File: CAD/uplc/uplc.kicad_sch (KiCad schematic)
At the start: 34 parts, among them J1 Conn_01x06_Pin, J2 SM12B-GHS-TB(LF)(SN), K1 G6K-2F-Y, K2 G6K-2F-Y, U1 DS8242-33S5, U3 ESP32-C3-WROOM-02, U5 TBD62003AFWG, Y1 32.568khz 3.2x1.5 12.5pf

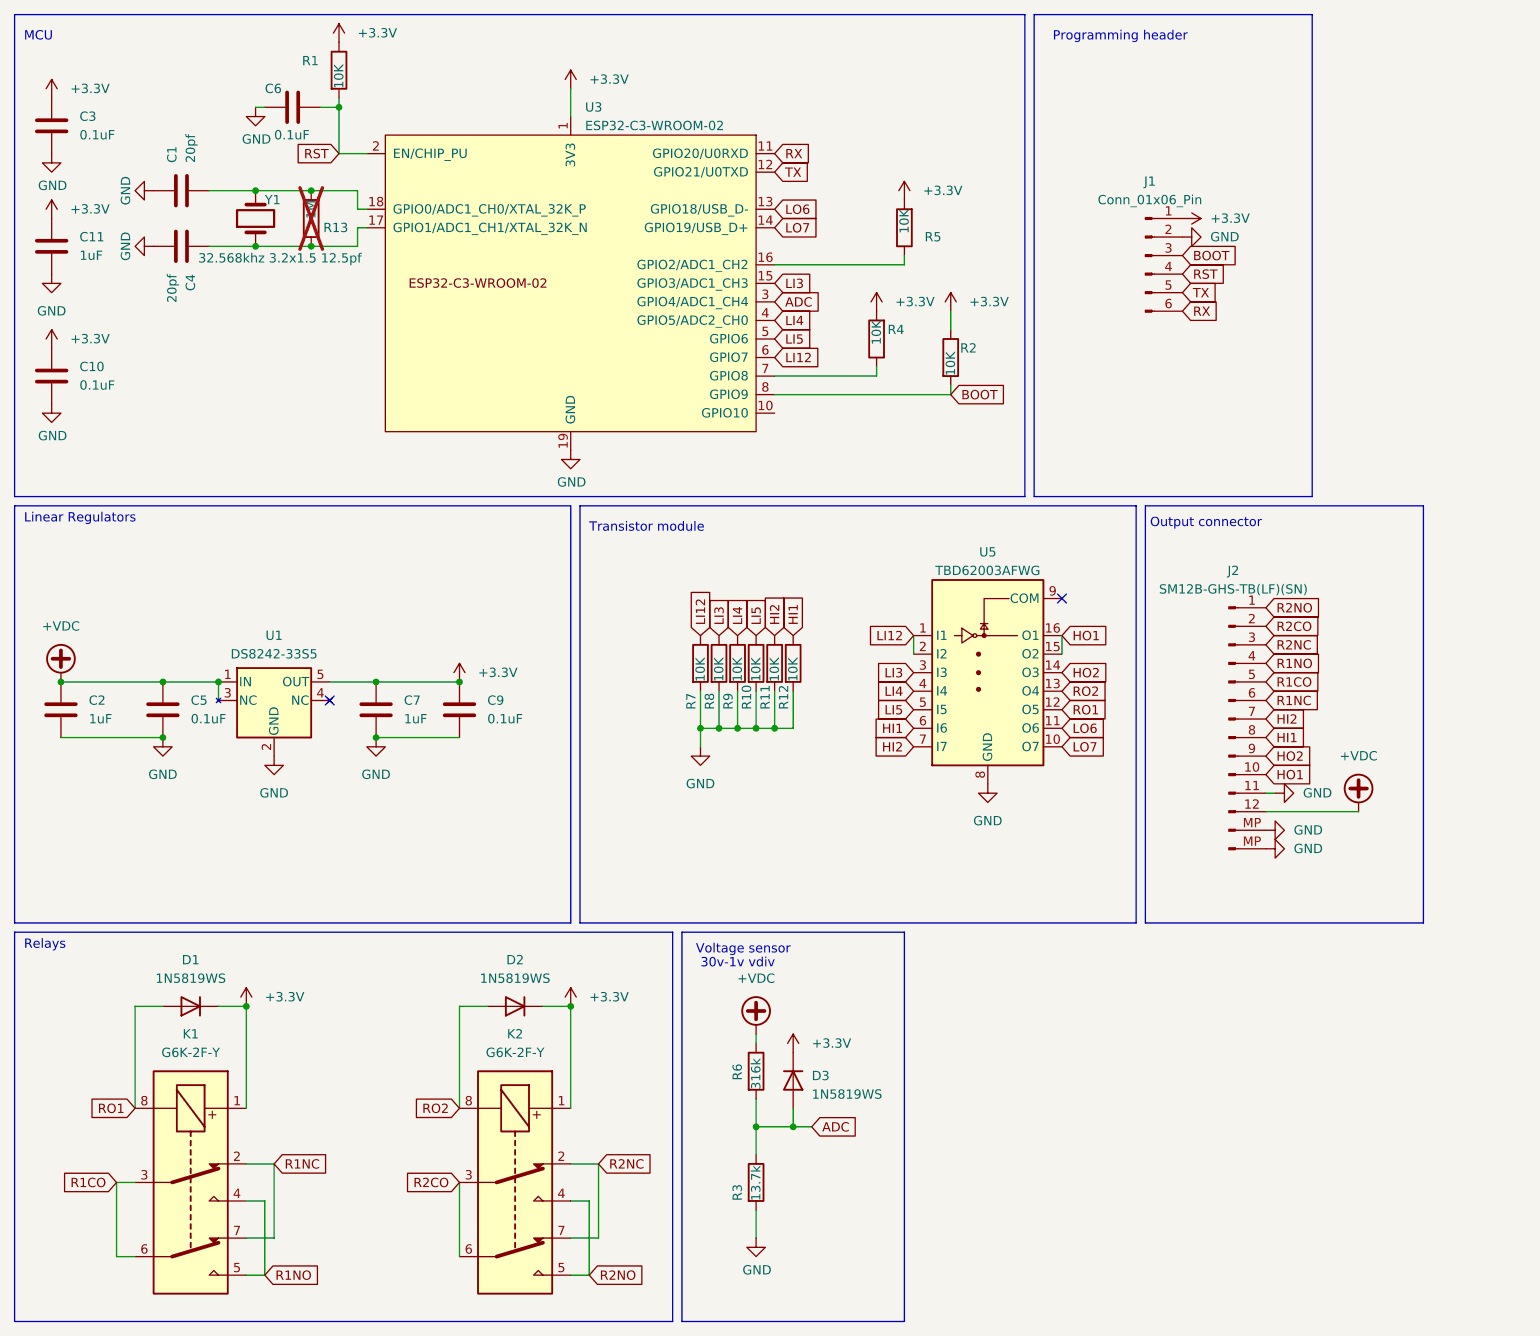
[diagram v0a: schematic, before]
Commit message: rev 1.1
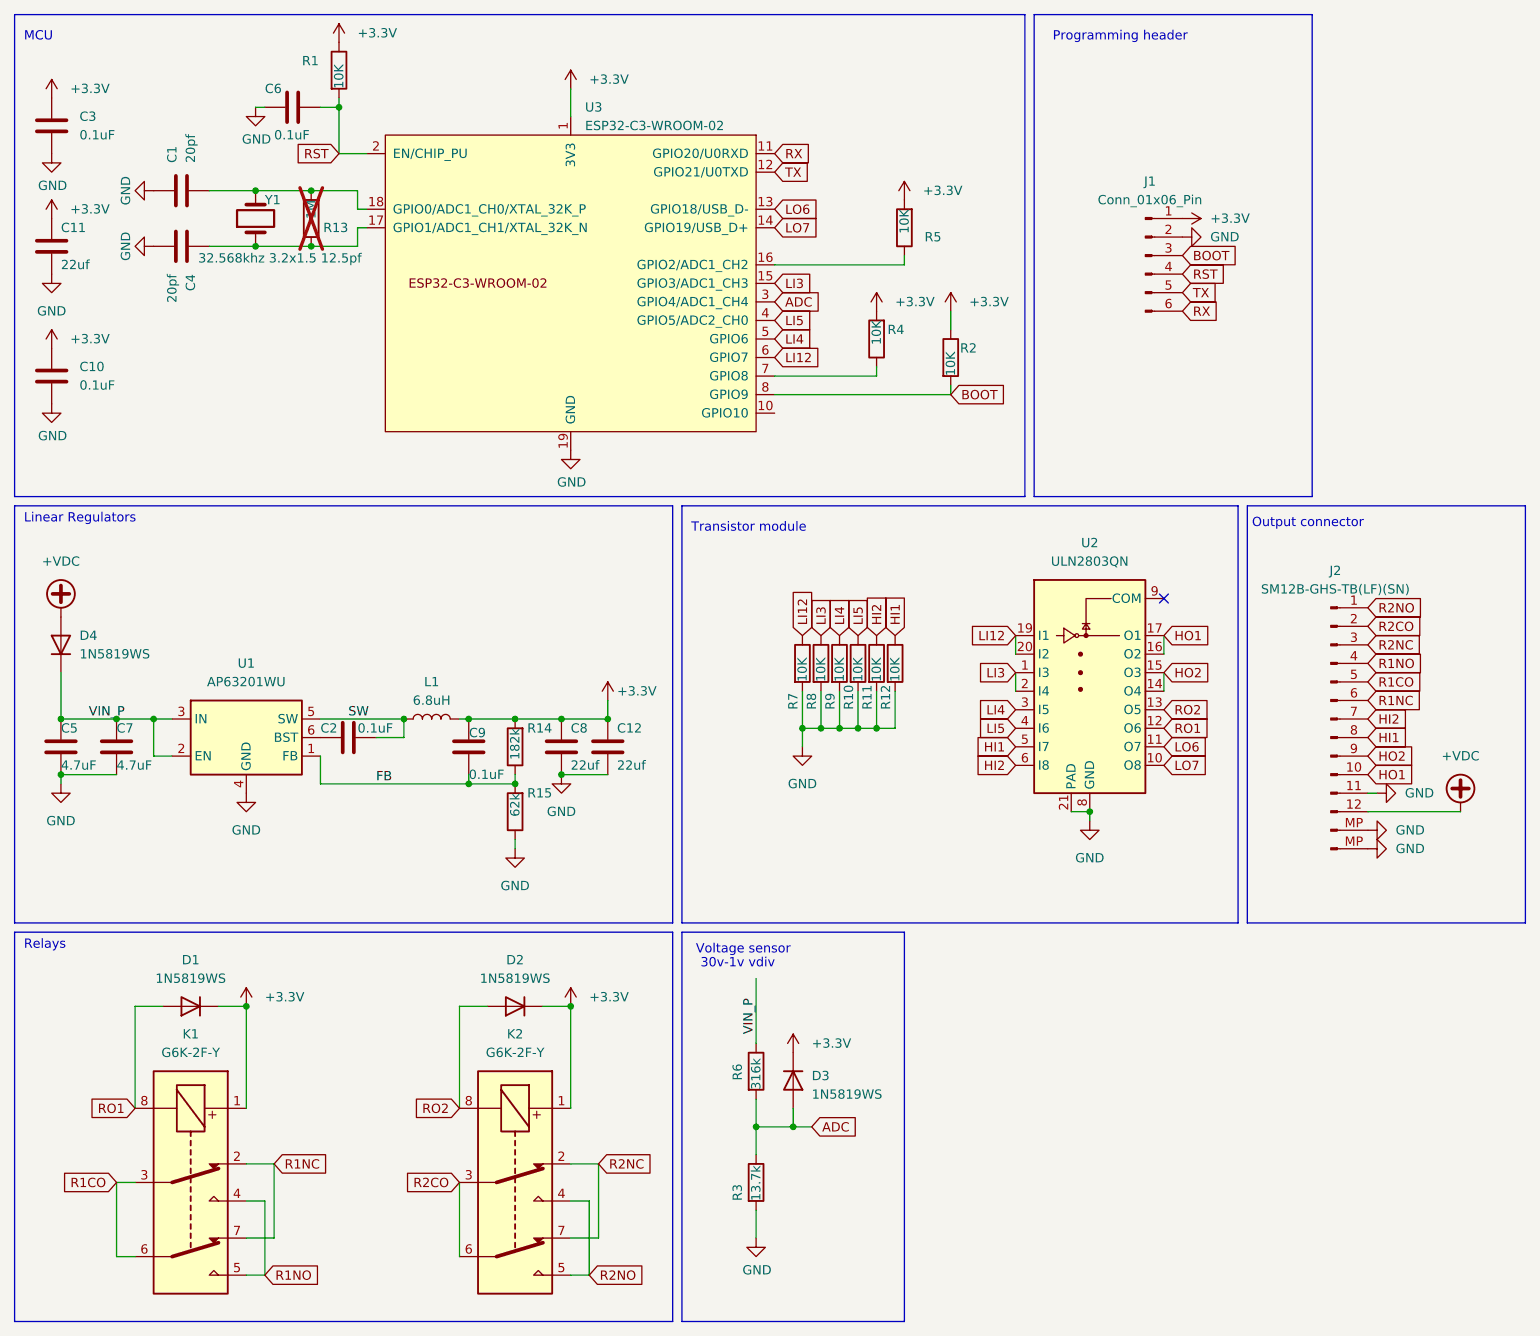
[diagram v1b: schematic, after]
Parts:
- removed U1: DS8242-33S5, Package_TO_SOT_SMD:SOT-23-5, symbol Library:DS8242
- removed U5: TBD62003AFWG, Package_SO:SOIC-16_3.9x9.9mm_P1.27mm, symbol Library:ULN2003A
- added C12, C8: 22uf, Capacitor_SMD:C_0402_1005Metric, symbol Library:C
- added D4: 1N5819WS, Diode_SMD:D_SOD-323, symbol Library:1N4148WS
- added L1: 6.8uH, Inductor_SMD:L_1008_2520Metric, symbol Device:L
- added R14: 182k, Resistor_SMD:R_0402_1005Metric, symbol Library:R
- added R15: 62k, Resistor_SMD:R_0402_1005Metric, symbol Library:R
- added U1: AP63201WU, Package_TO_SOT_SMD:TSOT-23-6, symbol Regulator_Switching:AP63201WU
- added U2: ULN2803QN, Package_DFN_QFN:QFN-20-1EP_4x4mm_P0.5mm_EP2.6x2.6mm, symbol Library:ULN2803QN
- C11: value 1uF -> 22uf; LCSC Part # C52923 -> C415703
- C2: value 1uF -> 0.1uF; LCSC Part # C52923 -> C307331
- C5: value 0.1uF -> 4.7uF; footprint Capacitor_SMD:C_0402_1005Metric -> Capacitor_SMD:C_0603_1608Metric
- C7: value 1uF -> 4.7uF; footprint Capacitor_SMD:C_0402_1005Metric -> Capacitor_SMD:C_0603_1608Metric; LCSC Part # C52923 -> C307331
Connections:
- net +3.3V: now also C12.1, C8.1, L1.2, R14.2; no longer C7.1
- net +VDC: now also D4.2 (A); no longer C2.1, C5.2, R6.1
- net GND: now also C5.2, C12.2, C8.2, R15.1, U1.4 (GND), U2.21 (PAD), U2.8 (GND); no longer C2.2, C5.1, C9.2
- net HI1: now also U2.5 (I7)
- net HI2: now also U2.6 (I8)
- net HO1: now also U2.16 (O2), U2.17 (O1)
- net HO2: now also U2.14 (O4), U2.15 (O3)
- net LI12: now also U2.19 (I1), U2.20 (I2)
- net LI3: now also U2.1 (I3), U2.2 (I4)
- net LI4: now also U3.5 (GPIO6), U2.3 (I5); no longer U3.4 (GPIO5/ADC2_CH0)
- net LI5: now also U3.4 (GPIO5/ADC2_CH0), U2.4 (I6); no longer U3.5 (GPIO6)
- net LO6: now also U2.11 (O7)
- net LO7: now also U2.10 (O8)
- net RO1: now also U2.12 (O6)
- net RO2: now also U2.13 (O5)
- new net: C2.2, U1.6 (BST)
- new net FB: C9.2, R14.1, R15.2, U1.1 (FB)
- new net SW: C2.1, L1.1, U1.5 (SW)
- new net VIN_P: C5.1, C7.1, D4.1 (K), R6.1, U1.2 (EN), U1.3 (IN)
- no-connect marks 2 -> 1
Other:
- moved on the sheet: J2, R10, R11, R12, R7, R8, R9

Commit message: Rev 1.2
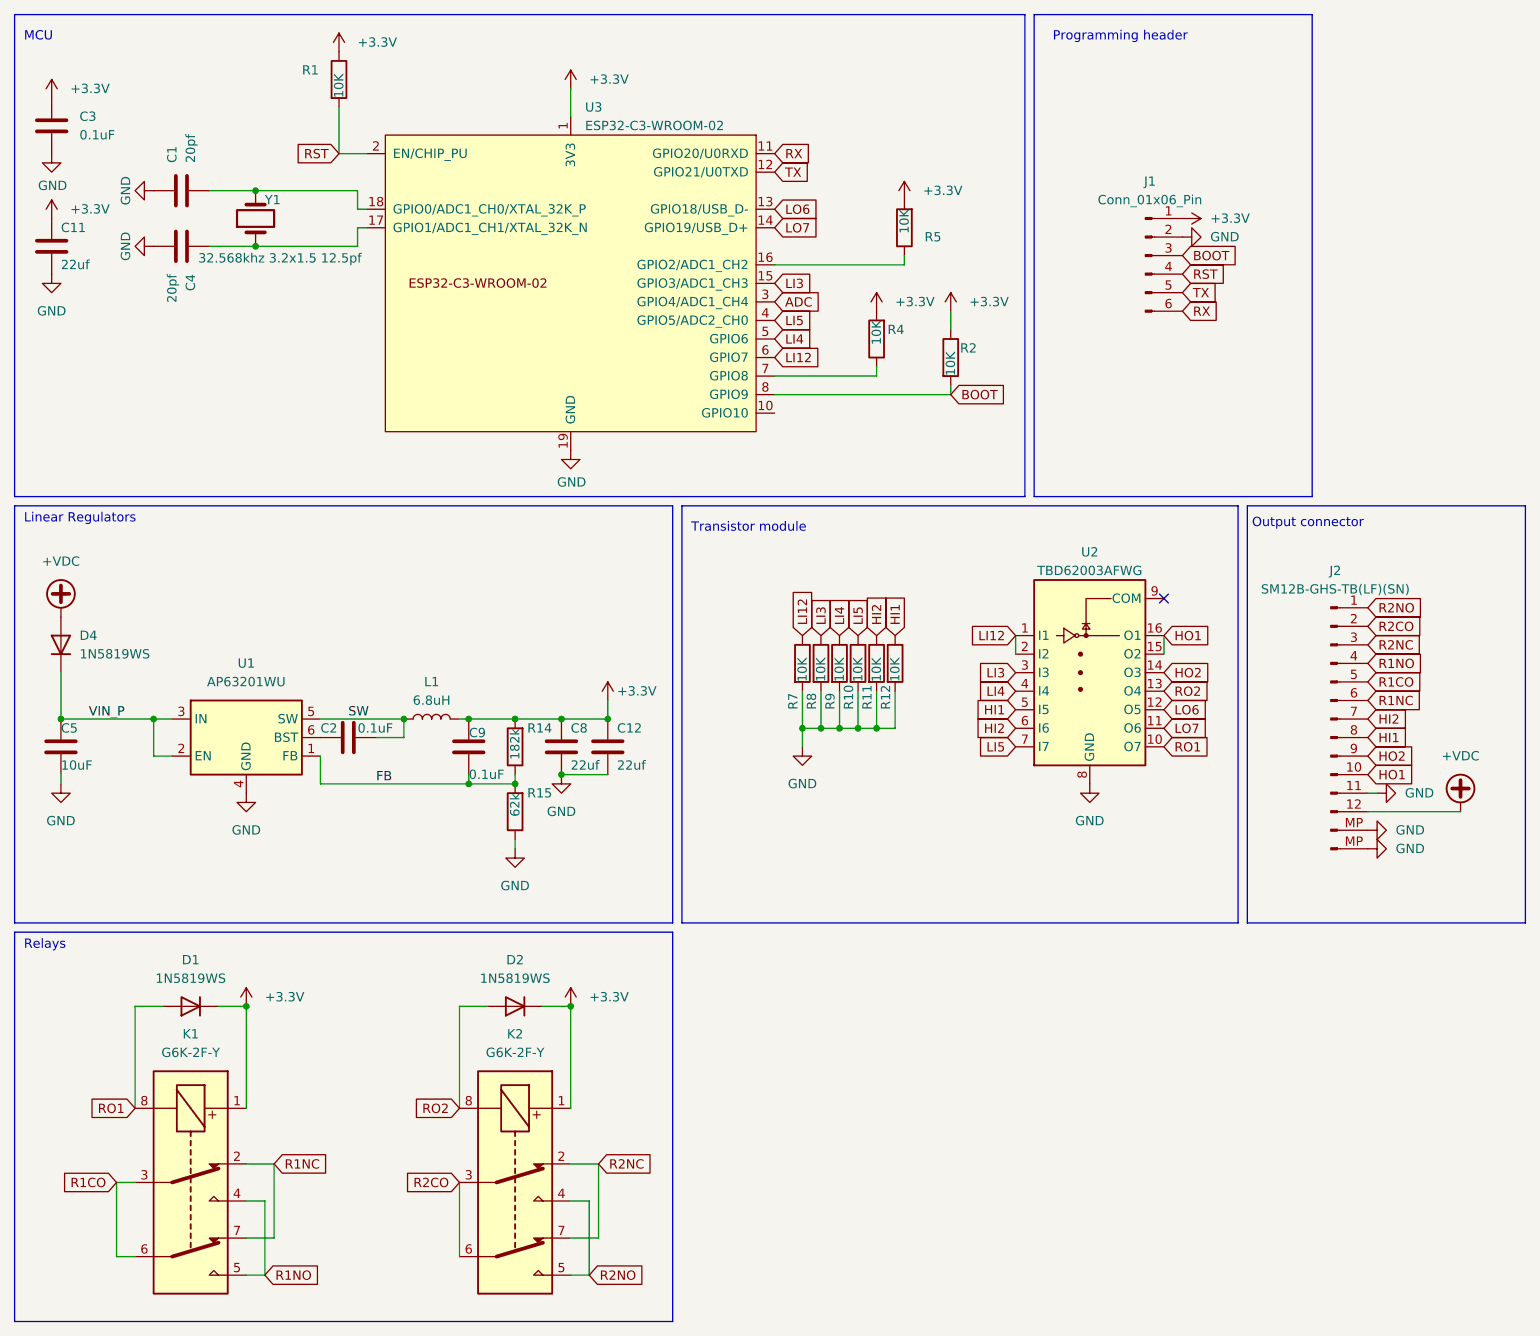
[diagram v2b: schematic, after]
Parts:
- removed C10, C6: 0.1uF, Capacitor_SMD:C_0402_1005Metric, symbol Library:C
- removed C7: 4.7uF, Capacitor_SMD:C_0603_1608Metric, symbol Library:C
- removed D3: 1N5819WS, Diode_SMD:D_SOD-323, symbol Library:1N4148WS
- removed R13: 1M, Resistor_SMD:R_0402_1005Metric, symbol Library:R
- removed R3: 13.7k, Resistor_SMD:R_0402_1005Metric, symbol Library:R
- removed R6: 316k, Resistor_SMD:R_0402_1005Metric, symbol Library:R
- removed U2: ULN2803QN, Package_DFN_QFN:QFN-20-1EP_4x4mm_P0.5mm_EP2.6x2.6mm, symbol Library:ULN2803QN
- added U2: TBD62003AFWG, Package_SO:SOIC-16_3.9x9.9mm_P1.27mm, symbol esprelay:ULN2003A
- C5: value 4.7uF -> 10uF; footprint Capacitor_SMD:C_0603_1608Metric -> Capacitor_SMD:C_0805_2012Metric; LCSC Part # C307331 -> (none)
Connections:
- net GND: now also U2.8 (GND)
- net HI1: now also U2.5 (I5)
- net HI2: now also U2.6 (I6)
- net HO1: now also U2.15 (O2), U2.16 (O1)
- net HO2: now also U2.14 (O3)
- net LI12: now also U2.1 (I1), U2.2 (I2)
- net LI3: now also U2.3 (I3)
- net LI4: now also U2.4 (I4)
- net LI5: now also U2.7 (I7)
- net LO6: now also U2.12 (O5)
- net LO7: now also U2.11 (O6)
- net RO1: now also U2.10 (O7)
- net RO2: now also U2.13 (O4)
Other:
- note removed: "30v-1v vdiv"
- note removed: "Voltage sensor"
- moved on the sheet: R1
